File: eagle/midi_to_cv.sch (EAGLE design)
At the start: 47 parts, among them IC2 4504N, IC3 4099N, U1 ATMEGA328P_PDIP

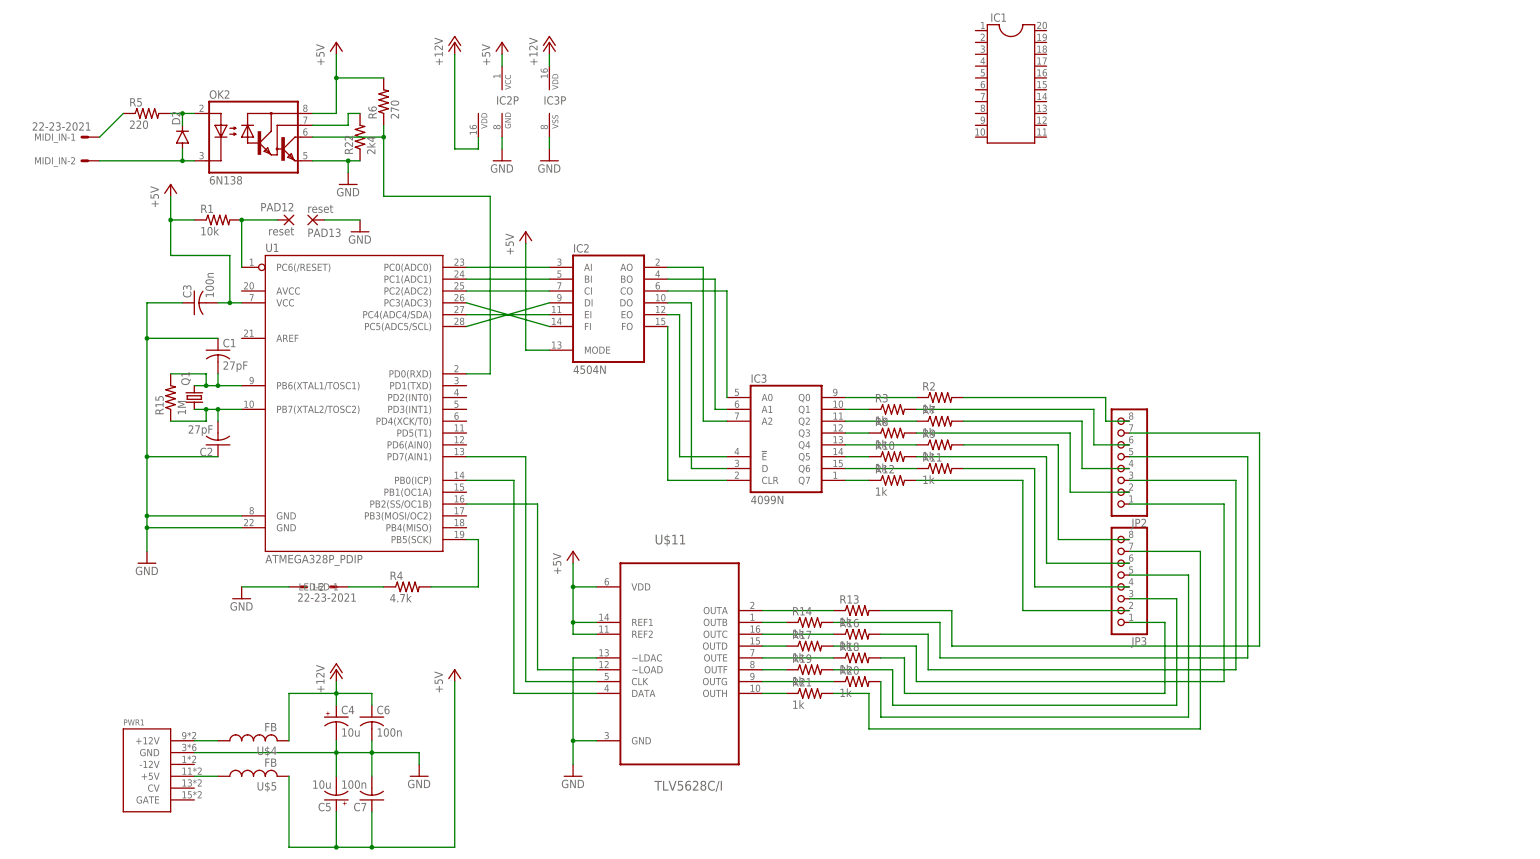
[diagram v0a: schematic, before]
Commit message: midi thru
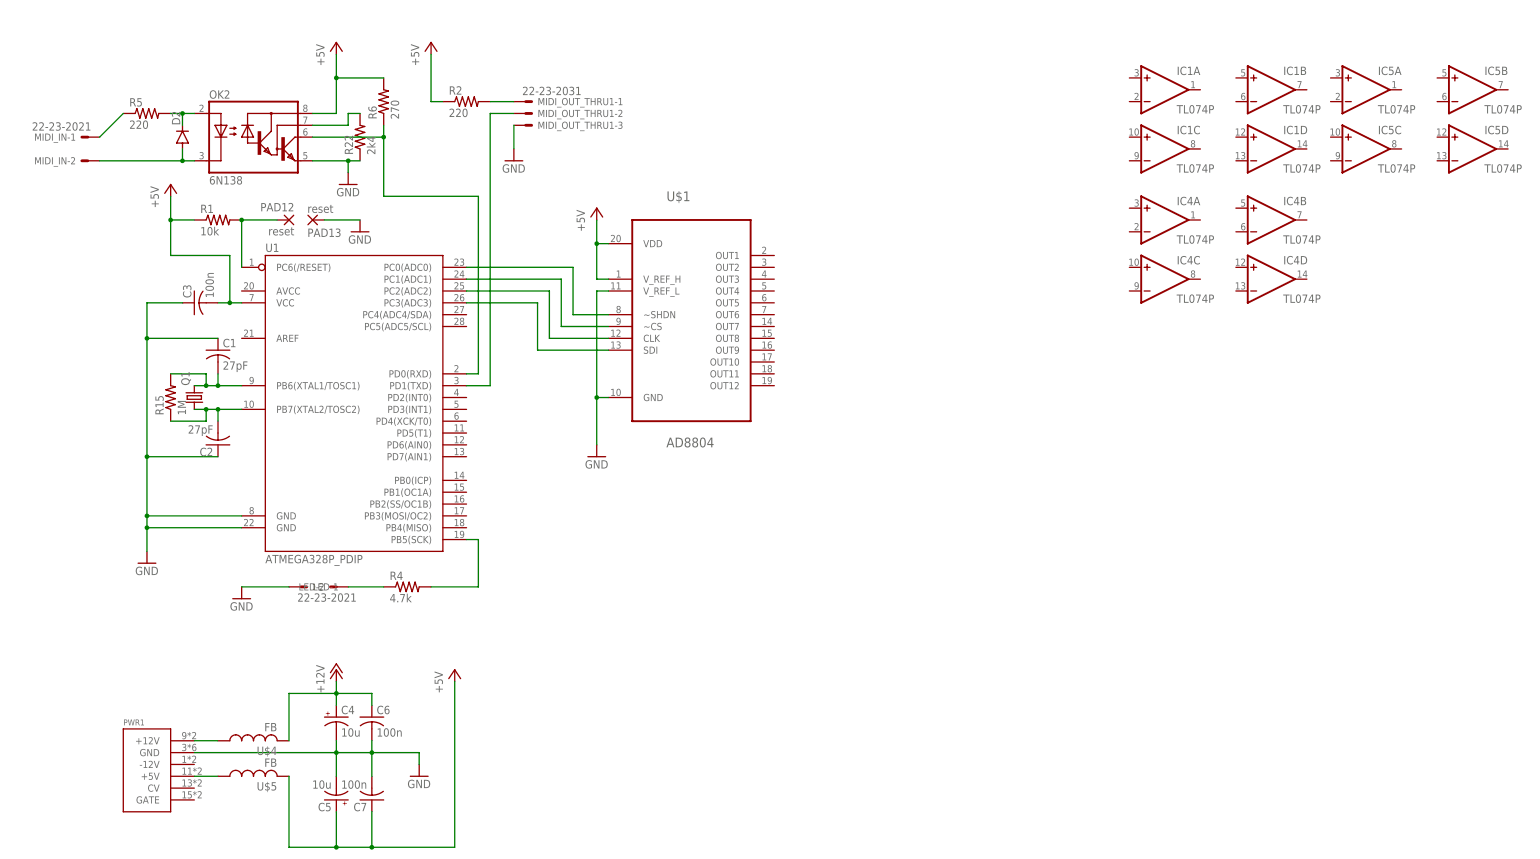
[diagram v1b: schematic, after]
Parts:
- removed IC2: 4504N, 45xx:4504N
- removed IC3: 4099N, 40xx:4099N
- removed JP2, JP3: (no value), pinhead:PINHD-1X8
- removed R10, R11, R12, R13, R14, R16, R17, R18, R19, R20, R21, R3, R7, R8, R9: 1k, rcl:R-US_0207/10
- removed U$11: TLV5628C/I, Texas Instruments_By_element14_Batch_1:TLV5628C/I
- added IC4, IC5: TL074P, linear:TL074P
- added MIDI_OUT_THRU1: 22-23-2031, con-molex:22-23-2031
- IC1: value (none) -> TL074P; device ic-package:DIL20 -> linear:TL074P
- R2: value 1k -> 220
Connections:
- removed net N$13: IC2A.CI, U1.PC2(ADC2)
- removed net N$14: U$11.CLK, U1.PD7(AIN1)
- removed net N$15: U$11.~LOAD, U1.PB2(SS/OC1B)
- removed net N$16: JP3.4, R11.2
- removed net N$21: JP3.2, R12.2
- removed net N$22: JP2.7, R13.2
- removed net N$23: IC2A.BI, U1.PC1(ADC1)
- removed net N$24: JP2.5, R14.2
- removed net N$25: IC2A.AI, U1.PC0(ADC0)
- removed net N$27: U$11.DATA, U1.PB0(ICP)
- removed net N$28: JP2.3, R16.2
- removed net N$29: JP2.1, R17.2
- removed net N$30: IC2A.DI, U1.PC5(ADC5/SCL)
- removed net N$31: IC2A.FI, U1.PC3(ADC3)
- removed net N$32: IC2A.EI, U1.PC4(ADC4/SDA)
- removed net N$33: IC2A.CO, IC3A.A0
- removed net N$34: JP3.5, R20.2
- removed net N$35: IC2A.BO, IC3A.A1
- removed net N$36: IC2A.AO, IC3A.A2
- removed net N$37: IC2A.DO, IC3A.D
- removed net N$38: IC2A.EO, IC3A.!E
- removed net N$39: IC3A.Q0, R2.1
- removed net N$40: JP3.1, R18.2
- removed net N$41: JP3.3, R19.2
- removed net N$44: IC3A.Q1, R3.1
- removed net N$45: IC3A.Q2, R7.1
- removed net N$46: IC3A.Q3, R8.1
- removed net N$47: IC3A.Q4, R9.1
- removed net N$48: IC3A.Q5, R10.1
- removed net N$49: IC3A.Q6, R11.1
- removed net N$50: IC3A.Q7, R12.1
- removed net N$51: JP3.7, R21.2
- removed net N$52: R13.1, U$11.OUTA
- removed net N$53: R14.1, U$11.OUTB
- removed net N$54: R16.1, U$11.OUTC
- removed net N$55: R17.1, U$11.OUTD
- removed net N$56: R18.1, U$11.OUTE
- removed net N$57: R19.1, U$11.OUTF
- removed net N$58: R20.1, U$11.OUTG
- removed net N$59: R21.1, U$11.OUTH
- removed net N$61: IC2A.FO, IC3A.CLR
- net +12V: no longer IC2P.VDD, IC3P.VDD
- net +5V: now also R2.1, U$1.VDD, U$1.V_REF_H; no longer IC2A.MODE, IC2P.VCC, U$11.REF1, U$11.REF2, U$11.VDD
- net GND: now also MIDI_OUT_THRU1-3.S, U$1.GND, U$1.V_REF_L; no longer IC2P.GND, IC3P.VSS, U$11.GND, U$11.~LDAC
- net N$12: now also MIDI_OUT_THRU1-2.S, U1.PD1(TXD); no longer JP3.6, R10.2
- net N$3: now also U$1.~SHDN, U1.PC0(ADC0); no longer JP2.8, R2.2
- net N$6: now also U$1.~CS, U1.PC1(ADC1); no longer JP2.6, R3.2
- net N$7: now also U$1.CLK, U1.PC2(ADC2); no longer JP2.4, R7.2
- net N$8: now also U$1.SDI, U1.PC3(ADC3); no longer JP2.2, R8.2
- net N$9: now also MIDI_OUT_THRU1-1.S, R2.2; no longer JP3.8, R9.2
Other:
- moved on the sheet: R2
